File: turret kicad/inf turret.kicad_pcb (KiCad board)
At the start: 2 copper layers, 45 x 45 mm, 27 parts, among them J1 Conn_01x06_Pin, J2 Conn_01x04_Pin, U1 XIAO-ESP32S3

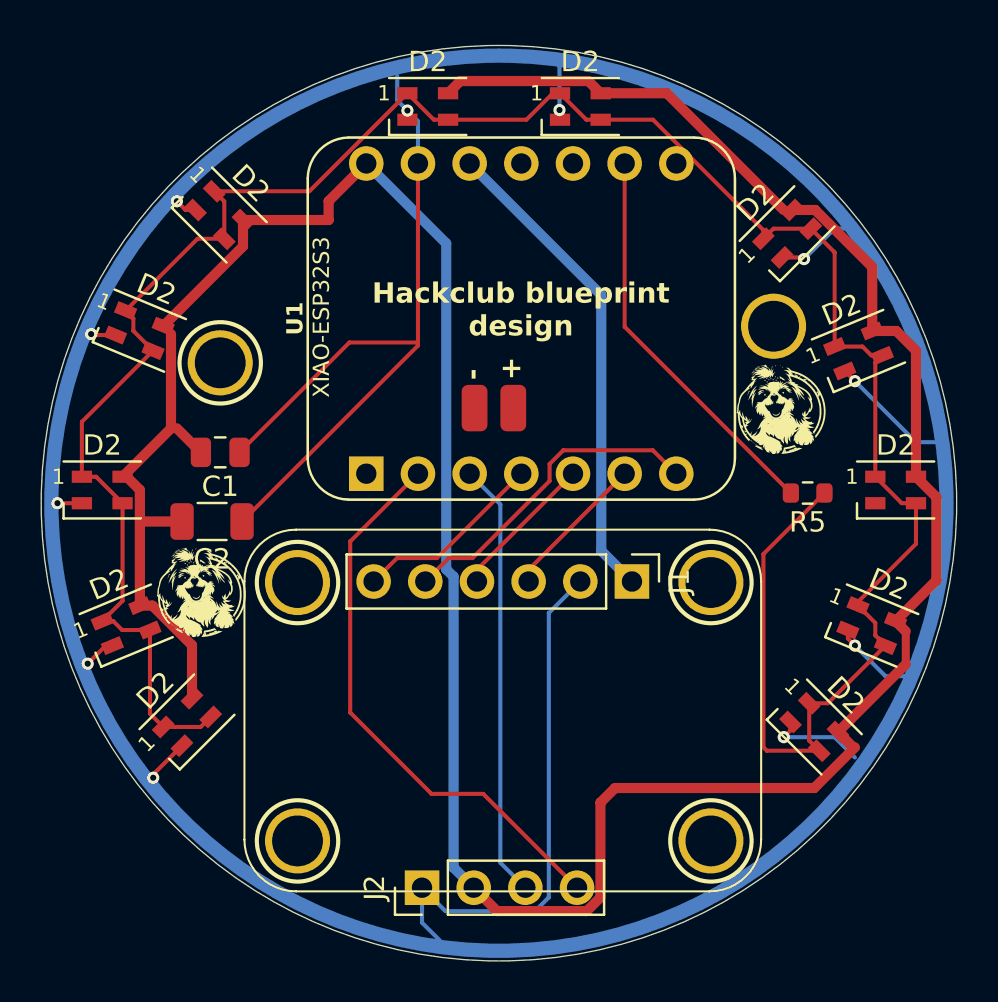
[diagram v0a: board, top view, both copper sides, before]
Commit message: update the design slightly
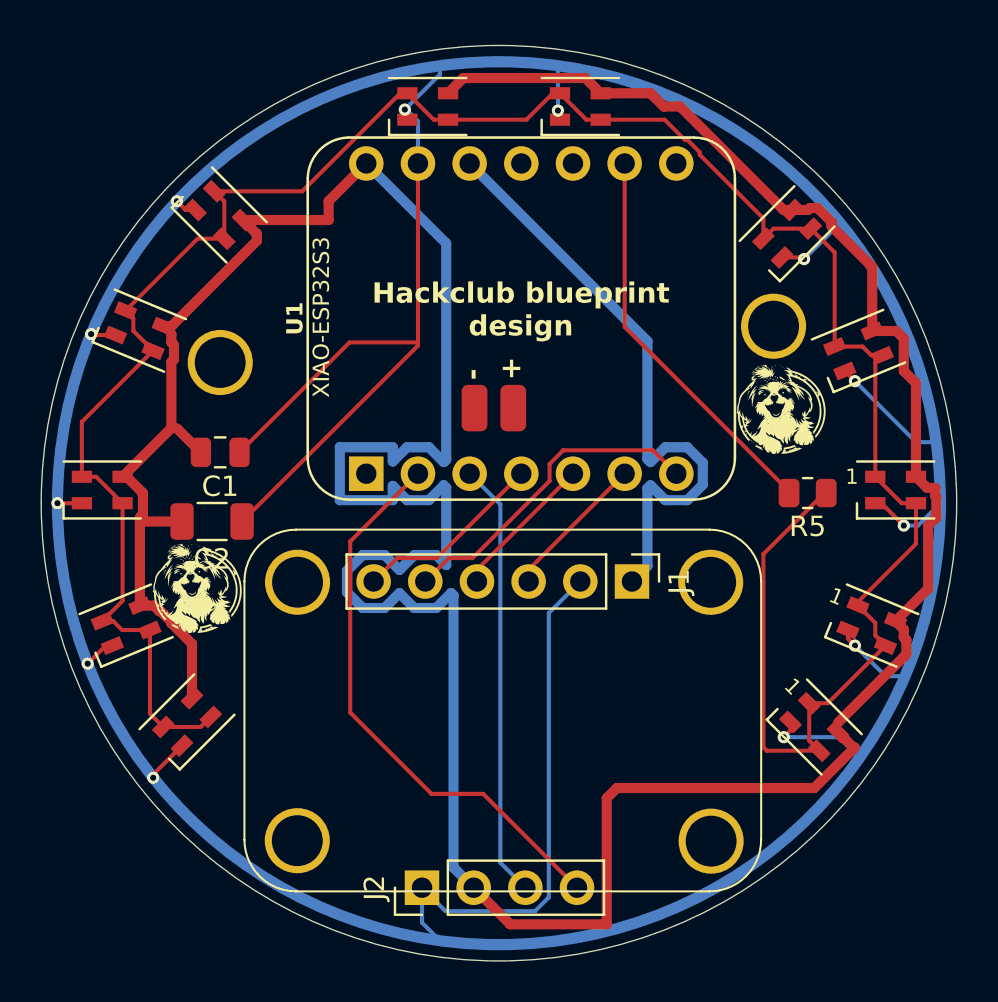
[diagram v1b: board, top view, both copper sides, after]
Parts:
- removed U$30, U$31, U$33 (x2), U$34: MOUNTINGHOLE2.5, Adafruit VL53L4CX:MOUNTINGHOLE_2.5_PLATED
- added ?: , , F.Cu at (157.9, 117.1)
- added ?: , , F.Cu at (133.8, 93.6)
- added ?: , , F.Cu at (157.9, 104.4)
- added ?: , , F.Cu at (137.6, 117.1)
- added ?: , , F.Cu at (137.6, 104.4)
- R5: footprint Resistor_SMD:R_0603_1608Metric -> Resistor_SMD:R_0805_2012Metric
- moved G*** 0.28 mm to (132.8, 104.8)
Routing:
- net +5V: track 156.4 -> 185.9 mm
- net VCC: track 24.0 -> 31.1 mm
- net GND: track 91.9 -> 97.9 mm, vias 11 -> 12
